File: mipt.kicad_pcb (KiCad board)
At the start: 2 copper layers, 1 part, among them U2 AW9523B

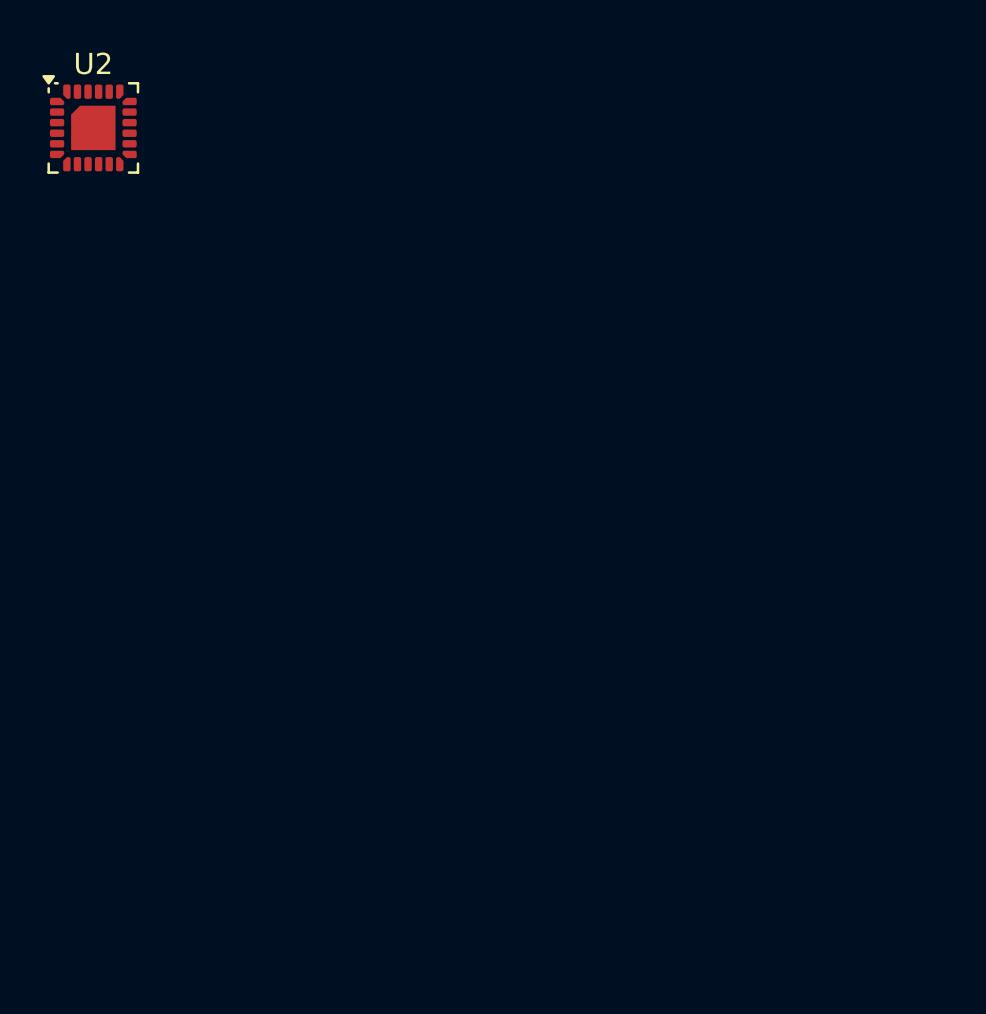
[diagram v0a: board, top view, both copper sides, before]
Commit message: some fixes
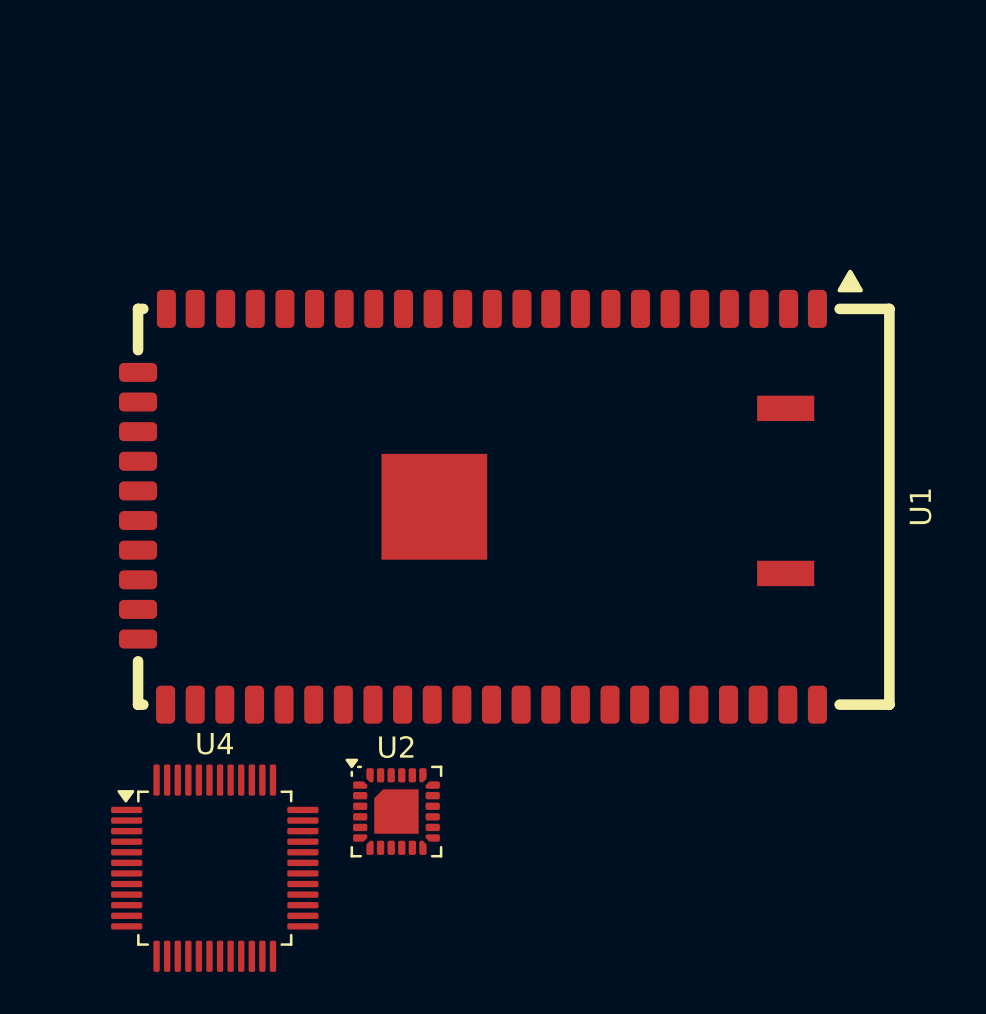
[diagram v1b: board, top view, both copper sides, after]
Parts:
- added U1: HLK-7628N, mipt:HLK-7628N, F.Cu at (67.2, 57.1)
- added U4: BL0910, Package_QFP:LQFP-48_7x7mm_P0.5mm, F.Cu at (53.0, 74.2)
- moved U2 35.3 mm to (61.6, 71.5)
